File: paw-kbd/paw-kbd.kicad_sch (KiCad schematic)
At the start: 62 parts, among them J1 OLED, J2 TRRS, J3 TRACKBALL, SW1 SW_PUSH, SW10 SW_PUSH, SW11 SW_PUSH, SW12 SW_PUSH, SW13 SW_PUSH, SW14 SW_PUSH, SW15 SW_PUSH, SW16 SW_PUSH, SW17 SW_PUSH, SW18 SW_PUSH, SW19 RotaryEncoder_Switch, SW2 SW_PUSH, SW3 SW_PUSH, SW4 SW_PUSH, SW5 SW_PUSH, SW6 SW_PUSH, SW7 SW_PUSH, SW8 SW_PUSH, SW9 SW_PUSH, U1 ProMicro

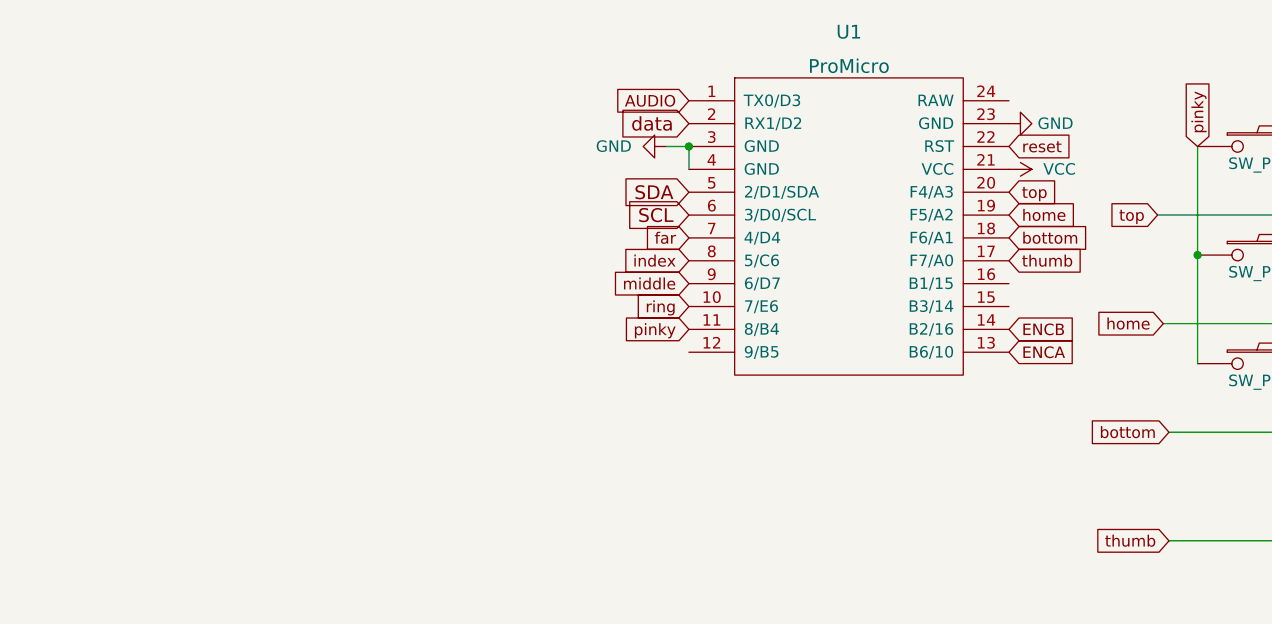
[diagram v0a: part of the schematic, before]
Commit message: seed
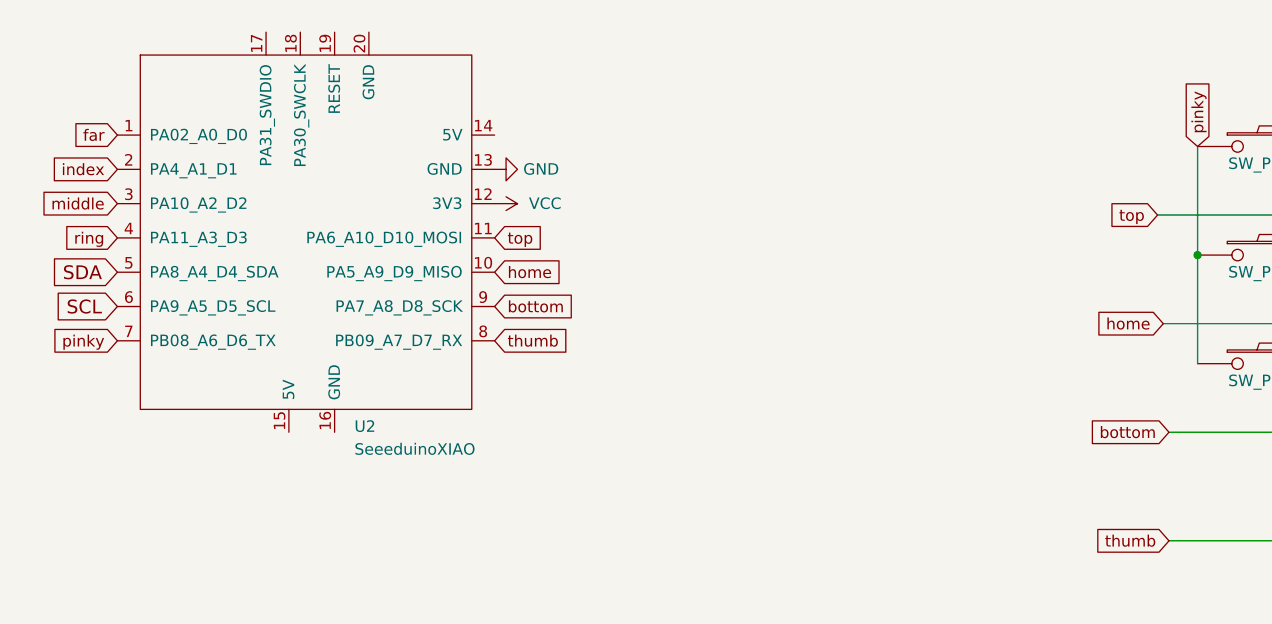
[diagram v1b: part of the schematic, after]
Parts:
- removed U1: ProMicro, keeb-footprints:ProMicro_v2, symbol kbd:ProMicro
- added U2: SeeeduinoXIAO, Seeeduino XIAO KICAD:Seeeduino XIAO-MOUDLE14P-2.54-21X17.8MM, symbol Seeeduino XIAO:SeeeduinoXIAO
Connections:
- net GND: now also U2.13 (GND)
- net SCL: now also U2.6 (PA9_A5_D5_SCL)
- net SDA: now also U2.5 (PA8_A4_D4_SDA)
- net VCC: now also U2.12 (3V3)
- net bottom: now also U2.9 (PA7_A8_D8_SCK)
- net far: now also U2.1 (PA02_A0_D0)
- net home: now also U2.10 (PA5_A9_D9_MISO)
- net index: now also U2.2 (PA4_A1_D1)
- net middle: now also U2.3 (PA10_A2_D2)
- net pinky: now also U2.7 (PB08_A6_D6_TX)
- net ring: now also U2.4 (PA11_A3_D3)
- net thumb: now also U2.8 (PB09_A7_D7_RX)
- net top: now also U2.11 (PA6_A10_D10_MOSI)
